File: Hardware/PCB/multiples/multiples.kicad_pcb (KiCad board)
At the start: 2 copper layers, 50 x 200 mm, 37 parts, among them J1 AudioJack2_SwitchT, J10 AudioJack2, J11 AudioJack2, J2 Synth_power_2x5, J3 AudioJack2, J4 AudioJack2, J5 AudioJack2, J6 AudioJack2, J7 AudioJack2_SwitchT, J8 AudioJack2, J9 AudioJack2, U1 TL074, U2 TL074

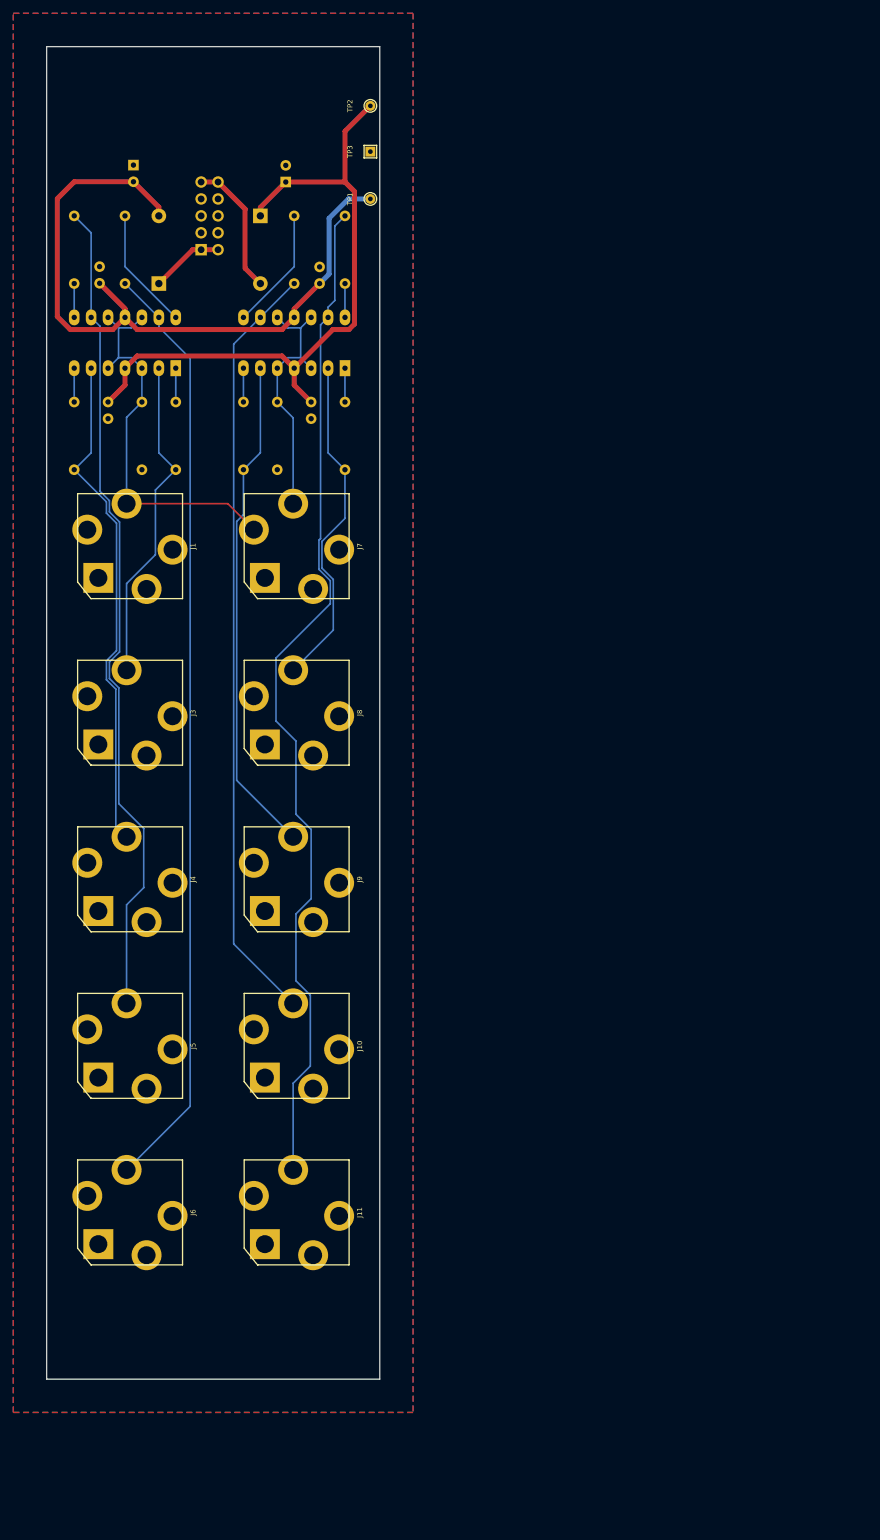
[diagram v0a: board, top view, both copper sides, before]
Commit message: KiCad 7, libraries to folder
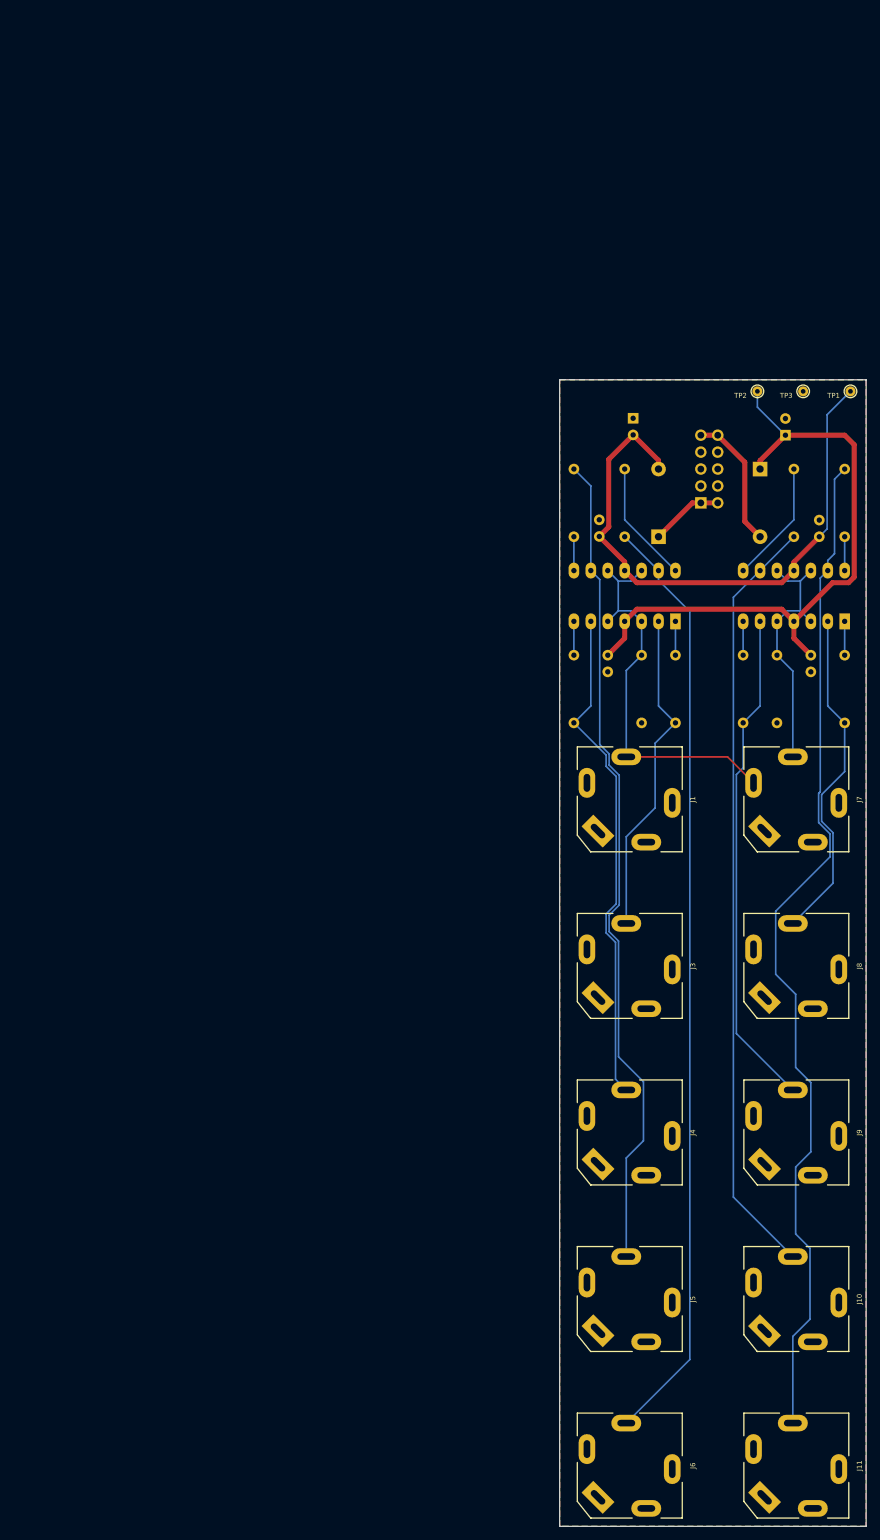
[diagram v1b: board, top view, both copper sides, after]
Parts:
- C1, C2: footprint ao_tht:CP_Radial_D6.3mm_P2.50mm -> AO_tht:CP_Radial_D6.3mm_P2.50mm
- C3, C4, C5, C6: footprint ao_tht:C_Disc_D3.0mm_W1.6mm_P2.50mm -> AO_tht:C_Disc_D3.0mm_W1.6mm_P2.50mm
- D1, D2: footprint ao_tht:D_DO-41_SOD81_P10.16mm_Horizontal -> AO_tht:D_DO-41_SOD81_P10.16mm_Horizontal
- GRAF2: footprint ao_tht:analogoutput -> AO_tht:analogoutput
- GRAF3: footprint ao_tht:CC0_logo -> AO_tht:CC0_logo
- J1, J10, J11, J3, J4, J5, J6, J7, J8, J9: footprint ao_tht:Jack_6.35mm_PJ_629HAN -> AO_tht:Jack_6.35mm_PJ_629HAN_slots
- J2: footprint ao_tht:Power_Header -> AO_tht:Power_Header
- R1, R10, R2, R3, R4, R5, R6, R7, R8, R9: footprint ao_tht:R_Axial_DIN0207_L6.3mm_D2.5mm_P10.16mm_Horizontal -> AO_tht:R_Axial_DIN0207_L6.3mm_D2.5mm_P10.16mm_Horizontal
- TP1, TP2: footprint ao_tht:TestPoint_THTPad_D1.5mm_Drill0.7mm -> AO_tht:TestPoint_THTPad_D1.5mm_Drill0.7mm
- TP3: footprint ao_tht:TestPoint_THTPad_1.5x1.5mm_Drill0.7mm -> AO_tht:TestPoint_THTPad_D1.5mm_Drill0.7mm
- U1, U2: footprint ao_tht:DIP-14_W7.62mm_Socket_LongPads -> AO_tht:DIP-14_W7.62mm_Socket_LongPads
- moved GRAF3 196.3 mm to (200.0, 180.0)
- moved R1 84.1 mm to (189.3, 91.3)
- moved C1 84.1 mm to (210.9, 58.3)
- moved C2 84.1 mm to (188.0, 55.8)
- moved C3 84.1 mm to (184.2, 91.3)
- moved C5 84.1 mm to (214.7, 91.3)
- moved C6 84.1 mm to (216.0, 71.1)
- moved D1 84.1 mm to (207.1, 63.4)
- moved D2 84.1 mm to (191.8, 73.6)
- moved GRAF1 84.1 mm to (200.0, 138.0)
- moved GRAF2 84.1 mm to (199.8, 126.3)
- moved J1 84.1 mm to (187.5, 113.0)
- moved J10 84.1 mm to (212.5, 188.0)
- moved J11 84.1 mm to (212.5, 213.0)
- moved J2 84.1 mm to (198.2, 68.5)
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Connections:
- J1 pad TN: GND -> (no net)
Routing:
- net -12V: track 106.6 -> 88.1 mm
- net +12V: track 101.4 -> 96.7 mm
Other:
- board size 50 x 200 mm -> 46 x 172.1 mm
- board text added: "Rich Holmes / Feb 2023 CC0 1.0 https://github.com/holmesrichards/mults"
- board text removed: "Rich Holmes / August 2021 CC0 1.0 https://github.com/holmesrichards/mults"
